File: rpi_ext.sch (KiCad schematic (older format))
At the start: 4 parts, among them J2 USB_OTG

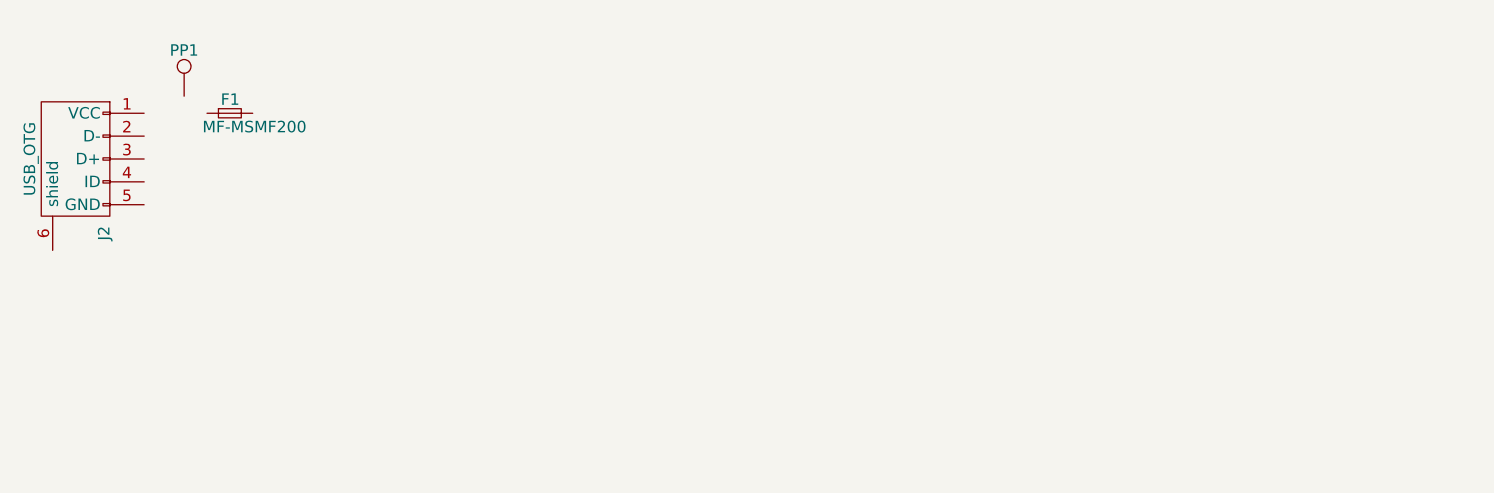
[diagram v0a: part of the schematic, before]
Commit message: update pdf
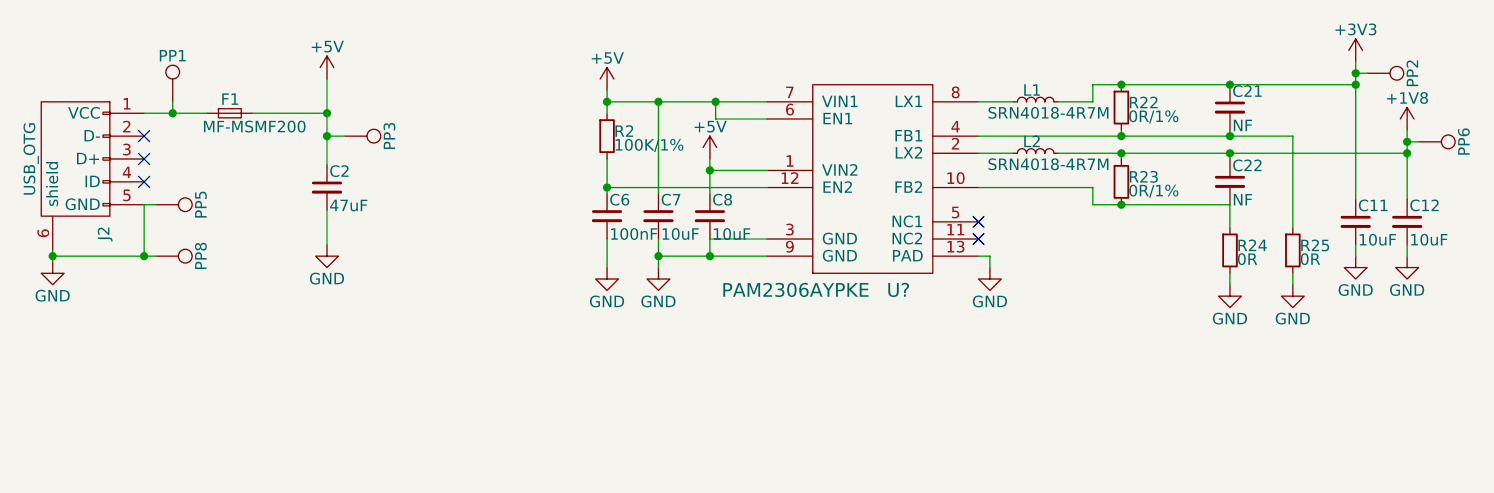
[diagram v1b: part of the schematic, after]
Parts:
- added C11, C12, C7, C8: 10uF, symbol C_Small
- added C2: 47uF, symbol C_Small
- added C21, C22: NF, symbol C_Small
- added C6: 100nF, symbol C_Small
- added L1, L2: SRN4018-4R7M, symbol L_Small
- added PP2, PP3, PP5, PP6, PP8: TEST_1P, symbol TEST_1P
- added R2: 100K/1%, symbol R_Small
- added R22, R23: 0R/1%, symbol R_Small
- added R24, R25: 0R, symbol R_Small
- added U?: PAM2306AYPKE, symbol PAM2306AYPKE
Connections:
- net at J2.1 (VCC): now also F1.1, PP1.1
- net GND: now reaches J2.5 (GND)
- net GND: now also J2.6 (shield), C11.2, C12.2, C2.2, C6.2, C7.2, C8.2, PP5.1, PP8.1, R24.2, R25.2, U?.13 (PAD), U?.3 (GND), U?.9 (GND)
- net +5V: now reaches F1.2
- net +5V: now also C2.1, C7.1, C8.1, PP3.1, R2.1, U?.1 (VIN2), U?.6 (EN1), U?.7 (VIN1)
- new net: C22.2, R23.2, R24.1, U?.10 (FB2)
- new net: C6.1, R2.2, U?.12 (EN2)
- new net: L2.1, U?.2 (LX2)
- new net: C21.2, R22.2, R25.1, U?.4 (FB1)
- new net: L1.1, U?.8 (LX1)
- new net +1V8: C12.1, C22.1, L2.2, PP6.1, R23.1
- new net +3V3: C11.1, C21.1, L1.2, PP2.1, R22.1
- no-connect marks 0 -> 5
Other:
- moved on the sheet: PP1
